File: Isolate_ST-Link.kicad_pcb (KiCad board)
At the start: 2 copper layers, 39 x 38 mm, 65 parts, among them J1 USB_OTG, J2 CONN_01X06, J3 CONN_01X04, J4 CONN_01X02, J5 CONN_01X02, J6 GS2, Q1 BSS138, U1 MAU10x, U2 ADuM4160, U3 APE8865NR-33-HF-3, U4 STM32F103CBTx, Y1 Crystal

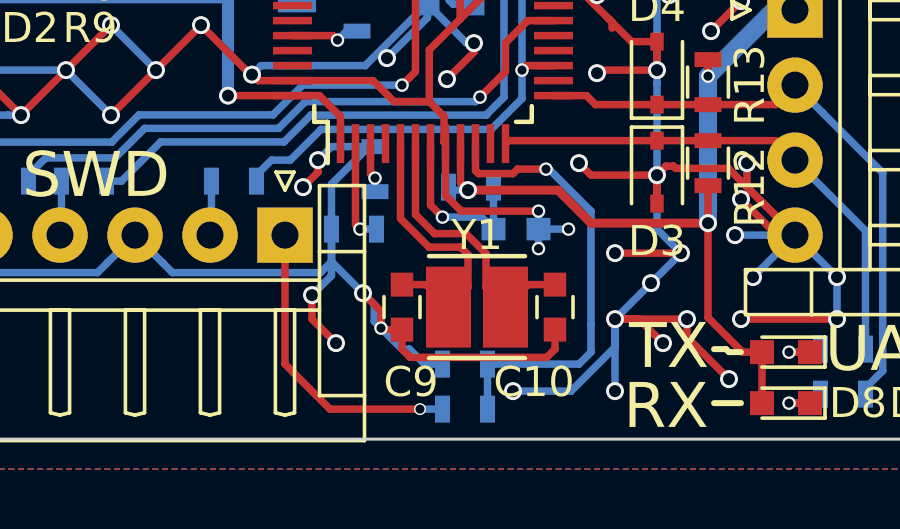
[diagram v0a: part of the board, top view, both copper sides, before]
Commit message: 配線の修正
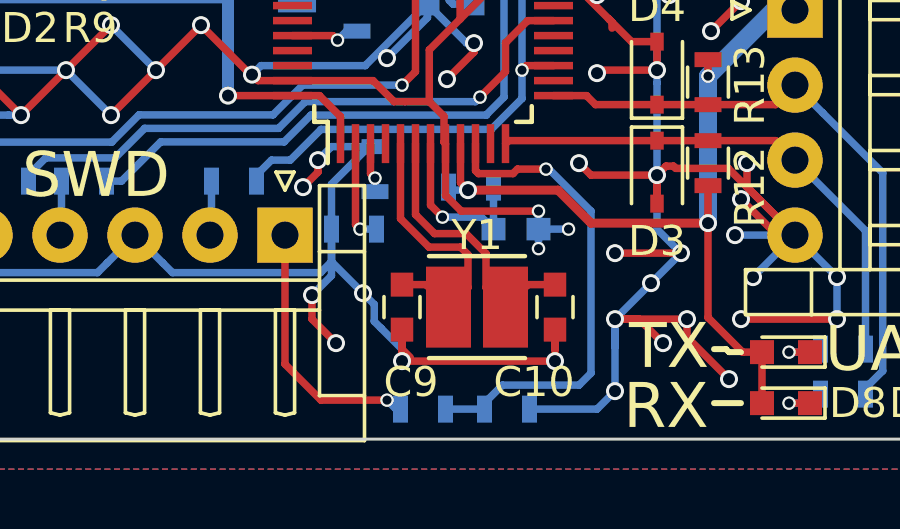
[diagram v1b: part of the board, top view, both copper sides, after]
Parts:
- moved R27 2.05 mm to (176.2, 87.0), turned to 0 degrees
- moved R29 1.40 mm to (173.4, 87.0)
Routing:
- net GND: track 389.6 -> 387.7 mm
- net /MCU/Vtarget: track 10.2 -> 8.77 mm
- net Net-(R27-Pad1): track 15.2 -> 16.3 mm
